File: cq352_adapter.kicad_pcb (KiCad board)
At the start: 2 copper layers, 2 parts, among them J1 FSI-150, X1 CQ352_SOCKET

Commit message: connector layout
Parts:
- added J2: FSI-150, spels:FSI-150-10-L-D-M-AD, F.Cu at (52.0, 135.0)
- added J3: FSI-150, spels:FSI-150-10-L-D-M-AD, F.Cu at (112.0, 205.0)
- added J4: FSI-150, spels:FSI-150-10-L-D-M-AD, F.Cu at (172.0, 135.0)
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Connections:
- J1 pad 1: Net-(J1-Pad1) -> (no net)
- J1 pad 10: Net-(J1-Pad10) -> (no net)
- J1 pad 100: Net-(J1-Pad100) -> (no net)
- J1 pad 11: Net-(J1-Pad11) -> (no net)
- J1 pad 12: Net-(J1-Pad12) -> (no net)
- J1 pad 13: Net-(J1-Pad13) -> (no net)
- J1 pad 14: Net-(J1-Pad14) -> (no net)
- J1 pad 15: Net-(J1-Pad15) -> (no net)
- J1 pad 16: Net-(J1-Pad16) -> (no net)
- J1 pad 17: Net-(J1-Pad17) -> (no net)
- J1 pad 18: Net-(J1-Pad18) -> (no net)
- J1 pad 19: Net-(J1-Pad19) -> (no net)
- J1 pad 2: Net-(J1-Pad2) -> (no net)
- J1 pad 20: Net-(J1-Pad20) -> (no net)
- J1 pad 21: Net-(J1-Pad21) -> (no net)
- J1 pad 22: Net-(J1-Pad22) -> (no net)
- J1 pad 23: Net-(J1-Pad23) -> (no net)
- J1 pad 24: Net-(J1-Pad24) -> (no net)
- J1 pad 25: Net-(J1-Pad25) -> (no net)
- J1 pad 26: Net-(J1-Pad26) -> (no net)
- J1 pad 27: Net-(J1-Pad27) -> (no net)
- J1 pad 28: Net-(J1-Pad28) -> (no net)
- J1 pad 29: Net-(J1-Pad29) -> (no net)
- J1 pad 3: Net-(J1-Pad3) -> (no net)
- J1 pad 30: Net-(J1-Pad30) -> (no net)
- J1 pad 31: Net-(J1-Pad31) -> (no net)
- J1 pad 32: Net-(J1-Pad32) -> (no net)
- J1 pad 33: Net-(J1-Pad33) -> (no net)
- J1 pad 34: Net-(J1-Pad34) -> (no net)
- J1 pad 35: Net-(J1-Pad35) -> (no net)
- J1 pad 36: Net-(J1-Pad36) -> (no net)
- J1 pad 37: Net-(J1-Pad37) -> (no net)
- J1 pad 38: Net-(J1-Pad38) -> (no net)
- J1 pad 39: Net-(J1-Pad39) -> (no net)
- J1 pad 4: Net-(J1-Pad4) -> (no net)
- J1 pad 40: Net-(J1-Pad40) -> (no net)
- J1 pad 41: Net-(J1-Pad41) -> (no net)
- J1 pad 42: Net-(J1-Pad42) -> (no net)
- J1 pad 43: Net-(J1-Pad43) -> (no net)
- J1 pad 44: Net-(J1-Pad44) -> (no net)
- J1 pad 45: Net-(J1-Pad45) -> (no net)
- J1 pad 46: Net-(J1-Pad46) -> (no net)
- J1 pad 47: Net-(J1-Pad47) -> (no net)
- J1 pad 48: Net-(J1-Pad48) -> (no net)
- J1 pad 49: Net-(J1-Pad49) -> (no net)
- J1 pad 5: Net-(J1-Pad5) -> (no net)
- J1 pad 50: Net-(J1-Pad50) -> (no net)
- J1 pad 51: Net-(J1-Pad51) -> (no net)
- J1 pad 52: Net-(J1-Pad52) -> (no net)
- J1 pad 53: Net-(J1-Pad53) -> (no net)
- J1 pad 54: Net-(J1-Pad54) -> (no net)
- J1 pad 55: Net-(J1-Pad55) -> (no net)
- J1 pad 56: Net-(J1-Pad56) -> (no net)
- J1 pad 57: Net-(J1-Pad57) -> (no net)
- J1 pad 58: Net-(J1-Pad58) -> (no net)
- J1 pad 59: Net-(J1-Pad59) -> (no net)
- J1 pad 6: Net-(J1-Pad6) -> (no net)
- J1 pad 60: Net-(J1-Pad60) -> (no net)
- J1 pad 61: Net-(J1-Pad61) -> (no net)
- J1 pad 62: Net-(J1-Pad62) -> (no net)
- J1 pad 63: Net-(J1-Pad63) -> (no net)
- J1 pad 64: Net-(J1-Pad64) -> (no net)
- J1 pad 65: Net-(J1-Pad65) -> (no net)
- J1 pad 66: Net-(J1-Pad66) -> (no net)
- J1 pad 67: Net-(J1-Pad67) -> (no net)
- J1 pad 68: Net-(J1-Pad68) -> (no net)
- J1 pad 69: Net-(J1-Pad69) -> (no net)
- J1 pad 7: Net-(J1-Pad7) -> (no net)
- J1 pad 70: Net-(J1-Pad70) -> (no net)
- J1 pad 71: Net-(J1-Pad71) -> (no net)
- J1 pad 72: Net-(J1-Pad72) -> (no net)
- J1 pad 73: Net-(J1-Pad73) -> (no net)
- J1 pad 74: Net-(J1-Pad74) -> (no net)
- J1 pad 75: Net-(J1-Pad75) -> (no net)
- J1 pad 76: Net-(J1-Pad76) -> (no net)
- J1 pad 77: Net-(J1-Pad77) -> (no net)
- J1 pad 78: Net-(J1-Pad78) -> (no net)
- J1 pad 79: Net-(J1-Pad79) -> (no net)
- J1 pad 8: Net-(J1-Pad8) -> (no net)
- J1 pad 80: Net-(J1-Pad80) -> (no net)
- J1 pad 81: Net-(J1-Pad81) -> (no net)
- J1 pad 82: Net-(J1-Pad82) -> (no net)
- J1 pad 83: Net-(J1-Pad83) -> (no net)
- J1 pad 84: Net-(J1-Pad84) -> (no net)
- J1 pad 85: Net-(J1-Pad85) -> (no net)
- J1 pad 86: Net-(J1-Pad86) -> (no net)
- J1 pad 87: Net-(J1-Pad87) -> (no net)
- J1 pad 88: Net-(J1-Pad88) -> (no net)
- J1 pad 89: Net-(J1-Pad89) -> (no net)
- J1 pad 9: Net-(J1-Pad9) -> (no net)
- J1 pad 90: Net-(J1-Pad90) -> (no net)
- J1 pad 91: Net-(J1-Pad91) -> (no net)
- J1 pad 92: Net-(J1-Pad92) -> (no net)
- J1 pad 93: Net-(J1-Pad93) -> (no net)
- J1 pad 94: Net-(J1-Pad94) -> (no net)
- J1 pad 95: Net-(J1-Pad95) -> (no net)
- J1 pad 96: Net-(J1-Pad96) -> (no net)
- J1 pad 97: Net-(J1-Pad97) -> (no net)
- J1 pad 98: Net-(J1-Pad98) -> (no net)
- J1 pad 99: Net-(J1-Pad99) -> (no net)
- J1 pad MH1: Net-(J1-PadMH1) -> (no net)
- J1 pad MH2: Net-(J1-PadMH2) -> (no net)
- J1 pad MH3: Net-(J1-PadMH3) -> (no net)
- X1 pad 1: Net-(X1-Pad1) -> (no net)
- X1 pad 10: Net-(X1-Pad10) -> (no net)
- X1 pad 100: Net-(X1-Pad100) -> (no net)
- X1 pad 101: Net-(X1-Pad101) -> (no net)
- X1 pad 102: Net-(X1-Pad102) -> (no net)
- X1 pad 103: Net-(X1-Pad103) -> (no net)
- X1 pad 104: Net-(X1-Pad104) -> (no net)
- X1 pad 105: Net-(X1-Pad105) -> (no net)
- X1 pad 106: Net-(X1-Pad106) -> (no net)
- X1 pad 107: Net-(X1-Pad107) -> (no net)
- X1 pad 108: Net-(X1-Pad108) -> (no net)
- X1 pad 109: Net-(X1-Pad109) -> (no net)
- X1 pad 11: Net-(X1-Pad11) -> (no net)
- X1 pad 110: Net-(X1-Pad110) -> (no net)
- X1 pad 111: Net-(X1-Pad111) -> (no net)
- X1 pad 112: Net-(X1-Pad112) -> (no net)
- X1 pad 113: Net-(X1-Pad113) -> (no net)
- X1 pad 114: Net-(X1-Pad114) -> (no net)
- X1 pad 115: Net-(X1-Pad115) -> (no net)
- X1 pad 116: Net-(X1-Pad116) -> (no net)
- X1 pad 117: Net-(X1-Pad117) -> (no net)
- X1 pad 118: Net-(X1-Pad118) -> (no net)
- X1 pad 119: Net-(X1-Pad119) -> (no net)
- X1 pad 12: Net-(X1-Pad12) -> (no net)
- X1 pad 120: Net-(X1-Pad120) -> (no net)
- X1 pad 121: Net-(X1-Pad121) -> (no net)
- X1 pad 122: Net-(X1-Pad122) -> (no net)
- X1 pad 123: Net-(X1-Pad123) -> (no net)
- X1 pad 124: Net-(X1-Pad124) -> (no net)
- X1 pad 125: Net-(X1-Pad125) -> (no net)
- X1 pad 126: Net-(X1-Pad126) -> (no net)
- X1 pad 127: Net-(X1-Pad127) -> (no net)
- X1 pad 128: Net-(X1-Pad128) -> (no net)
- X1 pad 129: Net-(X1-Pad129) -> (no net)
- X1 pad 13: Net-(X1-Pad13) -> (no net)
- X1 pad 130: Net-(X1-Pad130) -> (no net)
- X1 pad 131: Net-(X1-Pad131) -> (no net)
- X1 pad 132: Net-(X1-Pad132) -> (no net)
- X1 pad 133: Net-(X1-Pad133) -> (no net)
- X1 pad 134: Net-(X1-Pad134) -> (no net)
- X1 pad 135: Net-(X1-Pad135) -> (no net)
- X1 pad 136: Net-(X1-Pad136) -> (no net)
- X1 pad 137: Net-(X1-Pad137) -> (no net)
- X1 pad 138: Net-(X1-Pad138) -> (no net)
- X1 pad 139: Net-(X1-Pad139) -> (no net)
- X1 pad 14: Net-(X1-Pad14) -> (no net)
- X1 pad 140: Net-(X1-Pad140) -> (no net)
- X1 pad 141: Net-(X1-Pad141) -> (no net)
- X1 pad 142: Net-(X1-Pad142) -> (no net)
- X1 pad 143: Net-(X1-Pad143) -> (no net)
- X1 pad 144: Net-(X1-Pad144) -> (no net)
- X1 pad 145: Net-(X1-Pad145) -> (no net)
- X1 pad 146: Net-(X1-Pad146) -> (no net)
- X1 pad 147: Net-(X1-Pad147) -> (no net)
- X1 pad 148: Net-(X1-Pad148) -> (no net)
- X1 pad 149: Net-(X1-Pad149) -> (no net)
- X1 pad 15: Net-(X1-Pad15) -> (no net)
- X1 pad 150: Net-(X1-Pad150) -> (no net)
- X1 pad 151: Net-(X1-Pad151) -> (no net)
- X1 pad 152: Net-(X1-Pad152) -> (no net)
- X1 pad 153: Net-(X1-Pad153) -> (no net)
- X1 pad 154: Net-(X1-Pad154) -> (no net)
- X1 pad 155: Net-(X1-Pad155) -> (no net)
- X1 pad 156: Net-(X1-Pad156) -> (no net)
- X1 pad 157: Net-(X1-Pad157) -> (no net)
- X1 pad 158: Net-(X1-Pad158) -> (no net)
- X1 pad 159: Net-(X1-Pad159) -> (no net)
- X1 pad 16: Net-(X1-Pad16) -> (no net)
- X1 pad 160: Net-(X1-Pad160) -> (no net)
- X1 pad 161: Net-(X1-Pad161) -> (no net)
- X1 pad 162: Net-(X1-Pad162) -> (no net)
- X1 pad 163: Net-(X1-Pad163) -> (no net)
- X1 pad 164: Net-(X1-Pad164) -> (no net)
- X1 pad 165: Net-(X1-Pad165) -> (no net)
- X1 pad 166: Net-(X1-Pad166) -> (no net)
- X1 pad 167: Net-(X1-Pad167) -> (no net)
- X1 pad 168: Net-(X1-Pad168) -> (no net)
- X1 pad 169: Net-(X1-Pad169) -> (no net)
- X1 pad 17: Net-(X1-Pad17) -> (no net)
- X1 pad 170: Net-(X1-Pad170) -> (no net)
- X1 pad 171: Net-(X1-Pad171) -> (no net)
- X1 pad 172: Net-(X1-Pad172) -> (no net)
- X1 pad 173: Net-(X1-Pad173) -> (no net)
- X1 pad 174: Net-(X1-Pad174) -> (no net)
- X1 pad 175: Net-(X1-Pad175) -> (no net)
- X1 pad 176: Net-(X1-Pad176) -> (no net)
- X1 pad 177: Net-(X1-Pad177) -> (no net)
- X1 pad 178: Net-(X1-Pad178) -> (no net)
- X1 pad 179: Net-(X1-Pad179) -> (no net)
- X1 pad 18: Net-(X1-Pad18) -> (no net)
- X1 pad 180: Net-(X1-Pad180) -> (no net)
- X1 pad 181: Net-(X1-Pad181) -> (no net)
- X1 pad 182: Net-(X1-Pad182) -> (no net)
- X1 pad 183: Net-(X1-Pad183) -> (no net)
- X1 pad 184: Net-(X1-Pad184) -> (no net)
- X1 pad 185: Net-(X1-Pad185) -> (no net)
- X1 pad 186: Net-(X1-Pad186) -> (no net)
- X1 pad 187: Net-(X1-Pad187) -> (no net)
- X1 pad 188: Net-(X1-Pad188) -> (no net)
- X1 pad 189: Net-(X1-Pad189) -> (no net)
- X1 pad 19: Net-(X1-Pad19) -> (no net)
- X1 pad 190: Net-(X1-Pad190) -> (no net)
- X1 pad 191: Net-(X1-Pad191) -> (no net)
- X1 pad 192: Net-(X1-Pad192) -> (no net)
- X1 pad 193: Net-(X1-Pad193) -> (no net)
- X1 pad 194: Net-(X1-Pad194) -> (no net)
- X1 pad 195: Net-(X1-Pad195) -> (no net)
- X1 pad 196: Net-(X1-Pad196) -> (no net)
- X1 pad 197: Net-(X1-Pad197) -> (no net)
- X1 pad 198: Net-(X1-Pad198) -> (no net)
- X1 pad 199: Net-(X1-Pad199) -> (no net)
- X1 pad 2: Net-(X1-Pad2) -> (no net)
- X1 pad 20: Net-(X1-Pad20) -> (no net)
- X1 pad 200: Net-(X1-Pad200) -> (no net)
- X1 pad 201: Net-(X1-Pad201) -> (no net)
- X1 pad 202: Net-(X1-Pad202) -> (no net)
- X1 pad 203: Net-(X1-Pad203) -> (no net)
- X1 pad 204: Net-(X1-Pad204) -> (no net)
- X1 pad 205: Net-(X1-Pad205) -> (no net)
- X1 pad 206: Net-(X1-Pad206) -> (no net)
- X1 pad 207: Net-(X1-Pad207) -> (no net)
- X1 pad 208: Net-(X1-Pad208) -> (no net)
- X1 pad 209: Net-(X1-Pad209) -> (no net)
- X1 pad 21: Net-(X1-Pad21) -> (no net)
- X1 pad 210: Net-(X1-Pad210) -> (no net)
- X1 pad 211: Net-(X1-Pad211) -> (no net)
- X1 pad 212: Net-(X1-Pad212) -> (no net)
- X1 pad 213: Net-(X1-Pad213) -> (no net)
- X1 pad 214: Net-(X1-Pad214) -> (no net)
- X1 pad 215: Net-(X1-Pad215) -> (no net)
- X1 pad 216: Net-(X1-Pad216) -> (no net)
- X1 pad 217: Net-(X1-Pad217) -> (no net)
- X1 pad 218: Net-(X1-Pad218) -> (no net)
- X1 pad 219: Net-(X1-Pad219) -> (no net)
- X1 pad 22: Net-(X1-Pad22) -> (no net)
- X1 pad 220: Net-(X1-Pad220) -> (no net)
- X1 pad 221: Net-(X1-Pad221) -> (no net)
- X1 pad 222: Net-(X1-Pad222) -> (no net)
- X1 pad 223: Net-(X1-Pad223) -> (no net)
- X1 pad 224: Net-(X1-Pad224) -> (no net)
- X1 pad 225: Net-(X1-Pad225) -> (no net)
- X1 pad 226: Net-(X1-Pad226) -> (no net)
- X1 pad 227: Net-(X1-Pad227) -> (no net)
- X1 pad 228: Net-(X1-Pad228) -> (no net)
- X1 pad 229: Net-(X1-Pad229) -> (no net)
- X1 pad 23: Net-(X1-Pad23) -> (no net)
- X1 pad 230: Net-(X1-Pad230) -> (no net)
- X1 pad 231: Net-(X1-Pad231) -> (no net)
- X1 pad 232: Net-(X1-Pad232) -> (no net)
- X1 pad 233: Net-(X1-Pad233) -> (no net)
- X1 pad 234: Net-(X1-Pad234) -> (no net)
- X1 pad 235: Net-(X1-Pad235) -> (no net)
- X1 pad 236: Net-(X1-Pad236) -> (no net)
- X1 pad 237: Net-(X1-Pad237) -> (no net)
- X1 pad 238: Net-(X1-Pad238) -> (no net)
- X1 pad 239: Net-(X1-Pad239) -> (no net)
- X1 pad 24: Net-(X1-Pad24) -> (no net)
- X1 pad 240: Net-(X1-Pad240) -> (no net)
- X1 pad 241: Net-(X1-Pad241) -> (no net)
- X1 pad 242: Net-(X1-Pad242) -> (no net)
- X1 pad 243: Net-(X1-Pad243) -> (no net)
- X1 pad 244: Net-(X1-Pad244) -> (no net)
- X1 pad 245: Net-(X1-Pad245) -> (no net)
- X1 pad 246: Net-(X1-Pad246) -> (no net)
- X1 pad 247: Net-(X1-Pad247) -> (no net)
- X1 pad 248: Net-(X1-Pad248) -> (no net)
- X1 pad 249: Net-(X1-Pad249) -> (no net)
- X1 pad 25: Net-(X1-Pad25) -> (no net)
- X1 pad 250: Net-(X1-Pad250) -> (no net)
- X1 pad 251: Net-(X1-Pad251) -> (no net)
- X1 pad 252: Net-(X1-Pad252) -> (no net)
- X1 pad 253: Net-(X1-Pad253) -> (no net)
- X1 pad 254: Net-(X1-Pad254) -> (no net)
- X1 pad 255: Net-(X1-Pad255) -> (no net)
- X1 pad 256: Net-(X1-Pad256) -> (no net)
- X1 pad 257: Net-(X1-Pad257) -> (no net)
- X1 pad 258: Net-(X1-Pad258) -> (no net)
- X1 pad 259: Net-(X1-Pad259) -> (no net)
- X1 pad 26: Net-(X1-Pad26) -> (no net)
- X1 pad 260: Net-(X1-Pad260) -> (no net)
- X1 pad 261: Net-(X1-Pad261) -> (no net)
- X1 pad 262: Net-(X1-Pad262) -> (no net)
- X1 pad 263: Net-(X1-Pad263) -> (no net)
- X1 pad 264: Net-(X1-Pad264) -> (no net)
- X1 pad 265: Net-(X1-Pad265) -> (no net)
- X1 pad 266: Net-(X1-Pad266) -> (no net)
- X1 pad 267: Net-(X1-Pad267) -> (no net)
- X1 pad 268: Net-(X1-Pad268) -> (no net)
- X1 pad 269: Net-(X1-Pad269) -> (no net)
- X1 pad 27: Net-(X1-Pad27) -> (no net)
- X1 pad 270: Net-(X1-Pad270) -> (no net)
- X1 pad 271: Net-(X1-Pad271) -> (no net)
- X1 pad 272: Net-(X1-Pad272) -> (no net)
- X1 pad 273: Net-(X1-Pad273) -> (no net)
- X1 pad 274: Net-(X1-Pad274) -> (no net)
- X1 pad 275: Net-(X1-Pad275) -> (no net)
- X1 pad 276: Net-(X1-Pad276) -> (no net)
- X1 pad 277: Net-(X1-Pad277) -> (no net)
- X1 pad 278: Net-(X1-Pad278) -> (no net)
- X1 pad 279: Net-(X1-Pad279) -> (no net)
- X1 pad 28: Net-(X1-Pad28) -> (no net)
- X1 pad 280: Net-(X1-Pad280) -> (no net)
- X1 pad 281: Net-(X1-Pad281) -> (no net)
- X1 pad 282: Net-(X1-Pad282) -> (no net)
- X1 pad 283: Net-(X1-Pad283) -> (no net)
- X1 pad 284: Net-(X1-Pad284) -> (no net)
- X1 pad 285: Net-(X1-Pad285) -> (no net)
- X1 pad 286: Net-(X1-Pad286) -> (no net)
- X1 pad 287: Net-(X1-Pad287) -> (no net)
- X1 pad 288: Net-(X1-Pad288) -> (no net)
- X1 pad 289: Net-(X1-Pad289) -> (no net)
- X1 pad 29: Net-(X1-Pad29) -> (no net)
- X1 pad 290: Net-(X1-Pad290) -> (no net)
- X1 pad 291: Net-(X1-Pad291) -> (no net)
- X1 pad 292: Net-(X1-Pad292) -> (no net)
- X1 pad 293: Net-(X1-Pad293) -> (no net)
- X1 pad 294: Net-(X1-Pad294) -> (no net)
- X1 pad 295: Net-(X1-Pad295) -> (no net)
- X1 pad 296: Net-(X1-Pad296) -> (no net)
- X1 pad 297: Net-(X1-Pad297) -> (no net)
- X1 pad 298: Net-(X1-Pad298) -> (no net)
- X1 pad 299: Net-(X1-Pad299) -> (no net)
- X1 pad 3: Net-(X1-Pad3) -> (no net)
- X1 pad 30: Net-(X1-Pad30) -> (no net)
- X1 pad 300: Net-(X1-Pad300) -> (no net)
- X1 pad 301: Net-(X1-Pad301) -> (no net)
- X1 pad 302: Net-(X1-Pad302) -> (no net)
- X1 pad 303: Net-(X1-Pad303) -> (no net)
- X1 pad 304: Net-(X1-Pad304) -> (no net)
- X1 pad 305: Net-(X1-Pad305) -> (no net)
- X1 pad 306: Net-(X1-Pad306) -> (no net)
- X1 pad 307: Net-(X1-Pad307) -> (no net)
- X1 pad 308: Net-(X1-Pad308) -> (no net)
- X1 pad 309: Net-(X1-Pad309) -> (no net)
- X1 pad 31: Net-(X1-Pad31) -> (no net)
- X1 pad 310: Net-(X1-Pad310) -> (no net)
- X1 pad 311: Net-(X1-Pad311) -> (no net)
- X1 pad 312: Net-(X1-Pad312) -> (no net)
- X1 pad 313: Net-(X1-Pad313) -> (no net)
- X1 pad 314: Net-(X1-Pad314) -> (no net)
- X1 pad 315: Net-(X1-Pad315) -> (no net)
- X1 pad 316: Net-(X1-Pad316) -> (no net)
- X1 pad 317: Net-(X1-Pad317) -> (no net)
- X1 pad 318: Net-(X1-Pad318) -> (no net)
- X1 pad 319: Net-(X1-Pad319) -> (no net)
- X1 pad 32: Net-(X1-Pad32) -> (no net)
- X1 pad 320: Net-(X1-Pad320) -> (no net)
- X1 pad 321: Net-(X1-Pad321) -> (no net)
- X1 pad 322: Net-(X1-Pad322) -> (no net)
- X1 pad 323: Net-(X1-Pad323) -> (no net)
- X1 pad 324: Net-(X1-Pad324) -> (no net)
- X1 pad 325: Net-(X1-Pad325) -> (no net)
- X1 pad 326: Net-(X1-Pad326) -> (no net)
- X1 pad 327: Net-(X1-Pad327) -> (no net)
- X1 pad 328: Net-(X1-Pad328) -> (no net)
- X1 pad 329: Net-(X1-Pad329) -> (no net)
- X1 pad 33: Net-(X1-Pad33) -> (no net)
- X1 pad 330: Net-(X1-Pad330) -> (no net)
- X1 pad 331: Net-(X1-Pad331) -> (no net)
- X1 pad 332: Net-(X1-Pad332) -> (no net)
- X1 pad 333: Net-(X1-Pad333) -> (no net)
- X1 pad 334: Net-(X1-Pad334) -> (no net)
- X1 pad 335: Net-(X1-Pad335) -> (no net)
- X1 pad 336: Net-(X1-Pad336) -> (no net)
- X1 pad 337: Net-(X1-Pad337) -> (no net)
- X1 pad 338: Net-(X1-Pad338) -> (no net)
- X1 pad 339: Net-(X1-Pad339) -> (no net)
- X1 pad 34: Net-(X1-Pad34) -> (no net)
- X1 pad 340: Net-(X1-Pad340) -> (no net)
- X1 pad 341: Net-(X1-Pad341) -> (no net)
- X1 pad 342: Net-(X1-Pad342) -> (no net)
- X1 pad 343: Net-(X1-Pad343) -> (no net)
- X1 pad 344: Net-(X1-Pad344) -> (no net)
- X1 pad 345: Net-(X1-Pad345) -> (no net)
- X1 pad 346: Net-(X1-Pad346) -> (no net)
- X1 pad 347: Net-(X1-Pad347) -> (no net)
- X1 pad 348: Net-(X1-Pad348) -> (no net)
- X1 pad 349: Net-(X1-Pad349) -> (no net)
- X1 pad 35: Net-(X1-Pad35) -> (no net)
- X1 pad 350: Net-(X1-Pad350) -> (no net)
- X1 pad 351: Net-(X1-Pad351) -> (no net)
- X1 pad 352: Net-(X1-Pad352) -> (no net)
- X1 pad 36: Net-(X1-Pad36) -> (no net)
- X1 pad 37: Net-(X1-Pad37) -> (no net)
- X1 pad 38: Net-(X1-Pad38) -> (no net)
- X1 pad 39: Net-(X1-Pad39) -> (no net)
- X1 pad 4: Net-(X1-Pad4) -> (no net)
- X1 pad 40: Net-(X1-Pad40) -> (no net)
- X1 pad 41: Net-(X1-Pad41) -> (no net)
- X1 pad 42: Net-(X1-Pad42) -> (no net)
- X1 pad 43: Net-(X1-Pad43) -> (no net)
- X1 pad 44: Net-(X1-Pad44) -> (no net)
- X1 pad 45: Net-(X1-Pad45) -> (no net)
- X1 pad 46: Net-(X1-Pad46) -> (no net)
- X1 pad 47: Net-(X1-Pad47) -> (no net)
- X1 pad 48: Net-(X1-Pad48) -> (no net)
- X1 pad 49: Net-(X1-Pad49) -> (no net)
- X1 pad 5: Net-(X1-Pad5) -> (no net)
- X1 pad 50: Net-(X1-Pad50) -> (no net)
- X1 pad 51: Net-(X1-Pad51) -> (no net)
- X1 pad 52: Net-(X1-Pad52) -> (no net)
- X1 pad 53: Net-(X1-Pad53) -> (no net)
- X1 pad 54: Net-(X1-Pad54) -> (no net)
- X1 pad 55: Net-(X1-Pad55) -> (no net)
- X1 pad 56: Net-(X1-Pad56) -> (no net)
- X1 pad 57: Net-(X1-Pad57) -> (no net)
- X1 pad 58: Net-(X1-Pad58) -> (no net)
- X1 pad 59: Net-(X1-Pad59) -> (no net)
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
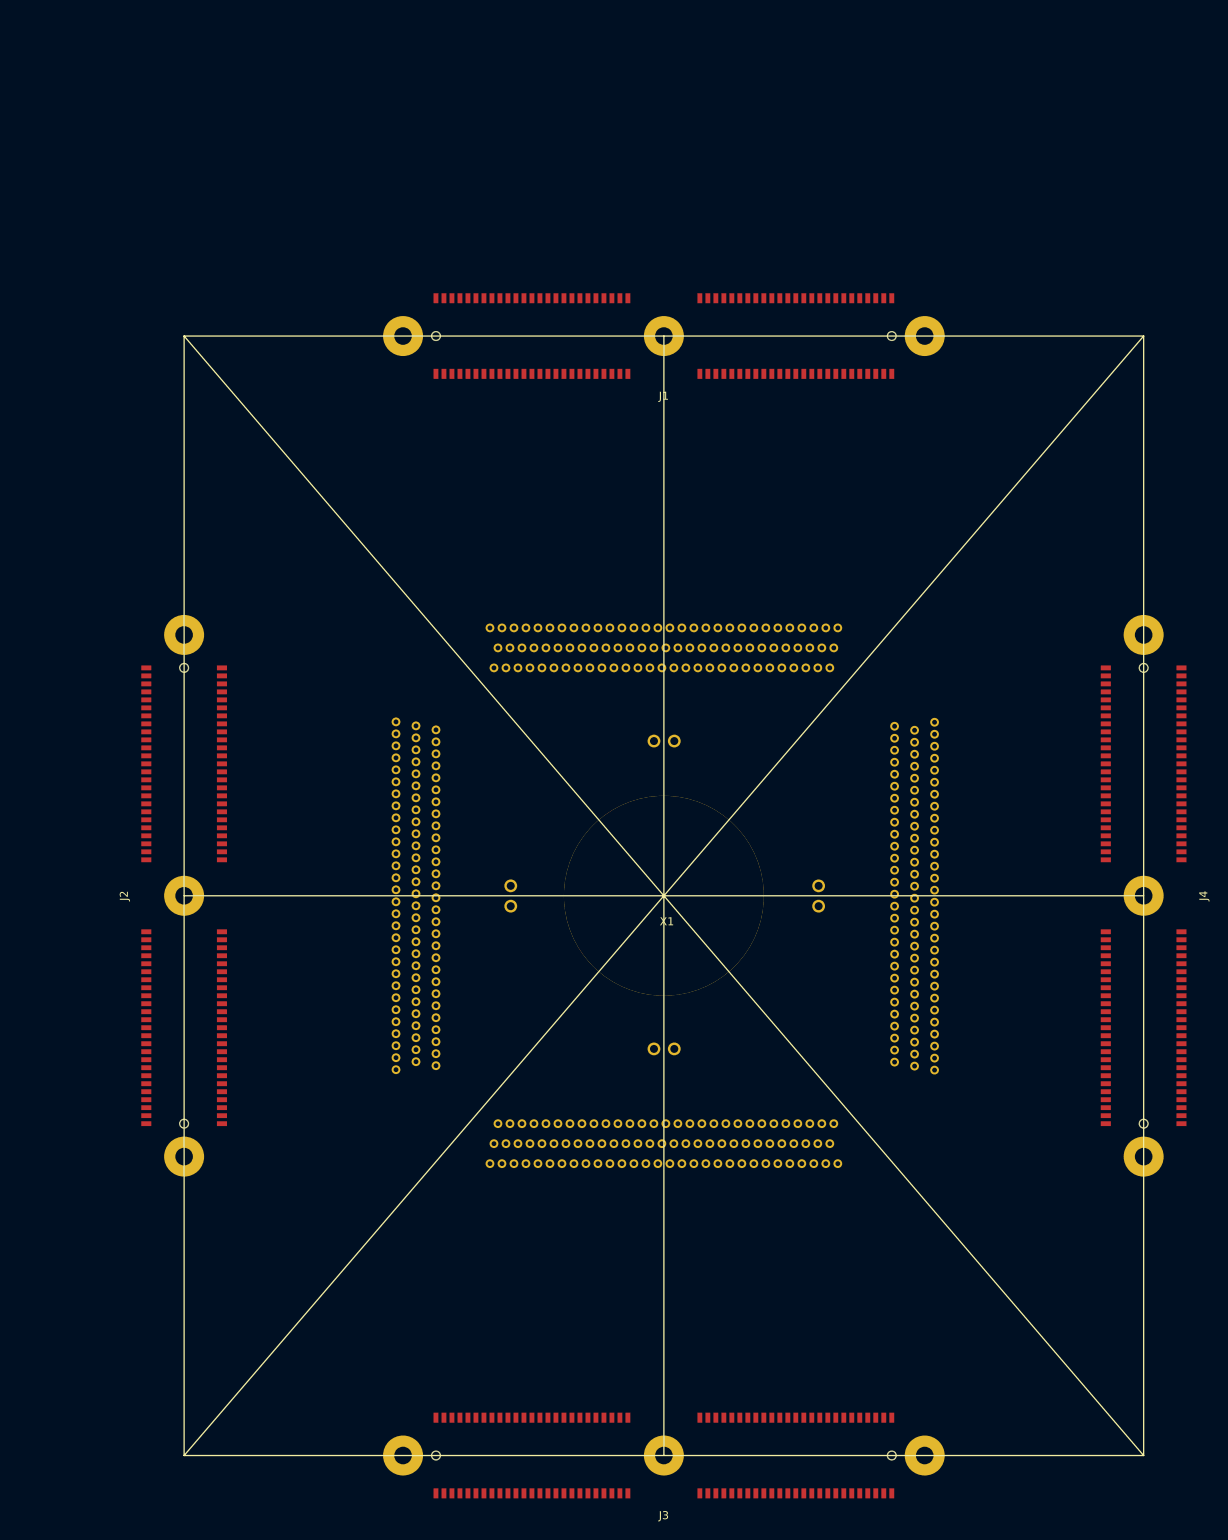
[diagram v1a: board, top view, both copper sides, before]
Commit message: routing signals
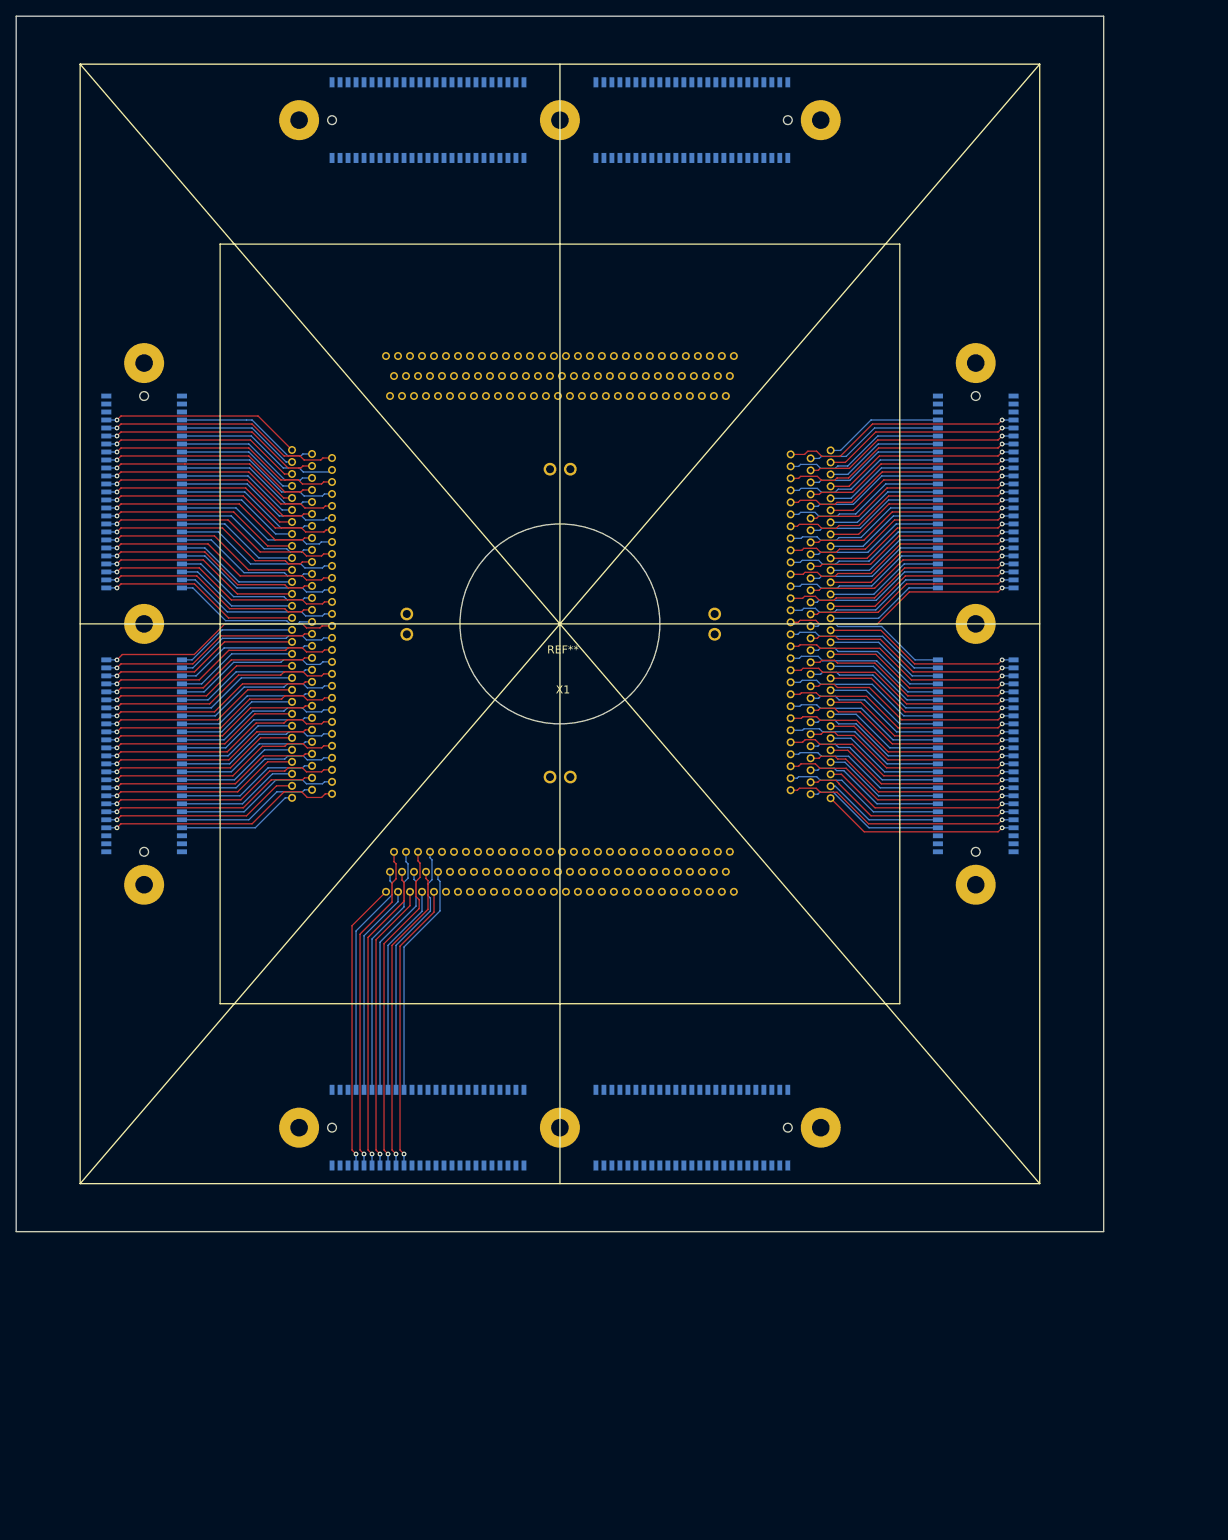
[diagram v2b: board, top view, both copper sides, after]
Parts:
- J1, J2, J3, J4: moved to B.Cu
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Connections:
- J1 pad 1: (no net) -> Net-(J1-Pad1)
- J1 pad 10: (no net) -> /4
- J1 pad 100: (no net) -> Net-(J1-Pad100)
- J1 pad 11: (no net) -> /5
- J1 pad 12: (no net) -> /6
- J1 pad 13: (no net) -> /7
- J1 pad 14: (no net) -> /8
- J1 pad 15: (no net) -> /9
- J1 pad 16: (no net) -> /10
- J1 pad 17: (no net) -> /11
- J1 pad 18: (no net) -> /12
- J1 pad 19: (no net) -> /13
- J1 pad 2: (no net) -> Net-(J1-Pad2)
- J1 pad 20: (no net) -> /14
- J1 pad 21: (no net) -> /15
- J1 pad 22: (no net) -> /16
- J1 pad 23: (no net) -> /17
- J1 pad 24: (no net) -> /18
- J1 pad 25: (no net) -> /19
- J1 pad 26: (no net) -> /20
- J1 pad 27: (no net) -> /21
- J1 pad 28: (no net) -> /22
- J1 pad 29: (no net) -> /23
- J1 pad 3: (no net) -> Net-(J1-Pad3)
- J1 pad 30: (no net) -> /24
- J1 pad 31: (no net) -> /25
- J1 pad 32: (no net) -> /26
- J1 pad 33: (no net) -> /27
- J1 pad 34: (no net) -> /28
- J1 pad 35: (no net) -> /29
- J1 pad 36: (no net) -> /30
- J1 pad 37: (no net) -> /31
- J1 pad 38: (no net) -> /32
- J1 pad 39: (no net) -> /33
- J1 pad 4: (no net) -> Net-(J1-Pad4)
- J1 pad 40: (no net) -> /34
- J1 pad 41: (no net) -> /35
- J1 pad 42: (no net) -> /36
- J1 pad 43: (no net) -> /37
- J1 pad 44: (no net) -> /38
- J1 pad 45: (no net) -> /39
- J1 pad 46: (no net) -> /40
- J1 pad 47: (no net) -> /41
- J1 pad 48: (no net) -> /42
- J1 pad 49: (no net) -> /43
- J1 pad 5: (no net) -> Net-(J1-Pad5)
- J1 pad 50: (no net) -> /44
- J1 pad 51: (no net) -> /45
- J1 pad 52: (no net) -> /46
- J1 pad 53: (no net) -> /47
- J1 pad 54: (no net) -> /48
- J1 pad 55: (no net) -> /49
- J1 pad 56: (no net) -> /50
- J1 pad 57: (no net) -> /51
- J1 pad 58: (no net) -> /52
- J1 pad 59: (no net) -> /53
- J1 pad 6: (no net) -> Net-(J1-Pad6)
- J1 pad 60: (no net) -> /54
- J1 pad 61: (no net) -> /55
- J1 pad 62: (no net) -> /56
- J1 pad 63: (no net) -> /57
- J1 pad 64: (no net) -> /58
- J1 pad 65: (no net) -> /59
- J1 pad 66: (no net) -> /60
- J1 pad 67: (no net) -> /61
- J1 pad 68: (no net) -> /62
- J1 pad 69: (no net) -> /63
- J1 pad 7: (no net) -> /1
- J1 pad 70: (no net) -> /64
- J1 pad 71: (no net) -> /65
- J1 pad 72: (no net) -> /66
- J1 pad 73: (no net) -> /67
- J1 pad 74: (no net) -> /68
- J1 pad 75: (no net) -> /69
- J1 pad 76: (no net) -> /70
- J1 pad 77: (no net) -> /71
- J1 pad 78: (no net) -> /72
- J1 pad 79: (no net) -> /73
- J1 pad 8: (no net) -> /2
- J1 pad 80: (no net) -> /74
- J1 pad 81: (no net) -> /75
- J1 pad 82: (no net) -> /76
- J1 pad 83: (no net) -> /77
- J1 pad 84: (no net) -> /78
- J1 pad 85: (no net) -> /79
- J1 pad 86: (no net) -> /80
- J1 pad 87: (no net) -> /81
- J1 pad 88: (no net) -> /82
- J1 pad 89: (no net) -> /83
- J1 pad 9: (no net) -> /3
- J1 pad 90: (no net) -> /84
- J1 pad 91: (no net) -> /85
- J1 pad 92: (no net) -> /86
- J1 pad 93: (no net) -> /87
- J1 pad 94: (no net) -> /88
- J1 pad 95: (no net) -> Net-(J1-Pad95)
- J1 pad 96: (no net) -> Net-(J1-Pad96)
- J1 pad 97: (no net) -> Net-(J1-Pad97)
- J1 pad 98: (no net) -> Net-(J1-Pad98)
- J1 pad 99: (no net) -> Net-(J1-Pad99)
- J1 pad MH1: (no net) -> Net-(J1-PadMH1)
- J1 pad MH2: (no net) -> Net-(J1-PadMH2)
- J1 pad MH3: (no net) -> Net-(J1-PadMH3)
- J2 pad 1: (no net) -> Net-(J2-Pad1)
- J2 pad 10: (no net) -> /92
- J2 pad 100: (no net) -> Net-(J2-Pad100)
- J2 pad 11: (no net) -> /93
- J2 pad 12: (no net) -> /94
- J2 pad 13: (no net) -> /95
- J2 pad 14: (no net) -> /96
- J2 pad 15: (no net) -> /97
- J2 pad 16: (no net) -> /98
- J2 pad 17: (no net) -> /99
- J2 pad 18: (no net) -> /100
- J2 pad 19: (no net) -> /101
- J2 pad 2: (no net) -> Net-(J2-Pad2)
- J2 pad 20: (no net) -> /102
- J2 pad 21: (no net) -> /103
- J2 pad 22: (no net) -> /104
- J2 pad 23: (no net) -> /105
- J2 pad 24: (no net) -> /106
- J2 pad 25: (no net) -> /107
- J2 pad 26: (no net) -> /108
- J2 pad 27: (no net) -> /109
- J2 pad 28: (no net) -> /110
- J2 pad 29: (no net) -> /111
- J2 pad 3: (no net) -> Net-(J2-Pad3)
- J2 pad 30: (no net) -> /112
- J2 pad 31: (no net) -> /113
- J2 pad 32: (no net) -> /114
- J2 pad 33: (no net) -> /115
- J2 pad 34: (no net) -> /116
- J2 pad 35: (no net) -> /117
- J2 pad 36: (no net) -> /118
- J2 pad 37: (no net) -> /119
- J2 pad 38: (no net) -> /120
- J2 pad 39: (no net) -> /121
- J2 pad 4: (no net) -> Net-(J2-Pad4)
- J2 pad 40: (no net) -> /122
- J2 pad 41: (no net) -> /123
- J2 pad 42: (no net) -> /124
- J2 pad 43: (no net) -> /125
- J2 pad 44: (no net) -> /126
- J2 pad 45: (no net) -> /127
- J2 pad 46: (no net) -> /128
- J2 pad 47: (no net) -> /129
- J2 pad 48: (no net) -> /130
- J2 pad 49: (no net) -> /131
- J2 pad 5: (no net) -> Net-(J2-Pad5)
- J2 pad 50: (no net) -> /132
- J2 pad 51: (no net) -> /133
- J2 pad 52: (no net) -> /134
- J2 pad 53: (no net) -> /135
- J2 pad 54: (no net) -> /136
- J2 pad 55: (no net) -> /137
- J2 pad 56: (no net) -> /138
- J2 pad 57: (no net) -> /139
- J2 pad 58: (no net) -> /140
- J2 pad 59: (no net) -> /141
- J2 pad 6: (no net) -> Net-(J2-Pad6)
- J2 pad 60: (no net) -> /142
- J2 pad 61: (no net) -> /143
- J2 pad 62: (no net) -> /144
- J2 pad 63: (no net) -> /145
- J2 pad 64: (no net) -> /146
- J2 pad 65: (no net) -> /147
- J2 pad 66: (no net) -> /148
- J2 pad 67: (no net) -> /149
- J2 pad 68: (no net) -> /150
- J2 pad 69: (no net) -> /151
- J2 pad 7: (no net) -> /89
- J2 pad 70: (no net) -> /152
- J2 pad 71: (no net) -> /153
- J2 pad 72: (no net) -> /154
- J2 pad 73: (no net) -> /155
- J2 pad 74: (no net) -> /156
- J2 pad 75: (no net) -> /157
- J2 pad 76: (no net) -> /158
- J2 pad 77: (no net) -> /159
- J2 pad 78: (no net) -> /160
- J2 pad 79: (no net) -> /161
- J2 pad 8: (no net) -> /90
- J2 pad 80: (no net) -> /162
- J2 pad 81: (no net) -> /163
- J2 pad 82: (no net) -> /164
- J2 pad 83: (no net) -> /165
- J2 pad 84: (no net) -> /166
- J2 pad 85: (no net) -> /167
- J2 pad 86: (no net) -> /168
- J2 pad 87: (no net) -> /169
- J2 pad 88: (no net) -> /170
- J2 pad 89: (no net) -> /171
- J2 pad 9: (no net) -> /91
- J2 pad 90: (no net) -> /172
- J2 pad 91: (no net) -> /173
- J2 pad 92: (no net) -> /174
- J2 pad 93: (no net) -> /175
- J2 pad 94: (no net) -> /176
- J2 pad 95: (no net) -> Net-(J2-Pad95)
- J2 pad 96: (no net) -> Net-(J2-Pad96)
- J2 pad 97: (no net) -> Net-(J2-Pad97)
- J2 pad 98: (no net) -> Net-(J2-Pad98)
- J2 pad 99: (no net) -> Net-(J2-Pad99)
- J2 pad MH1: (no net) -> Net-(J2-PadMH1)
- J2 pad MH2: (no net) -> Net-(J2-PadMH2)
- J2 pad MH3: (no net) -> Net-(J2-PadMH3)
- J3 pad 1: (no net) -> Net-(J3-Pad1)
- J3 pad 10: (no net) -> /180
- J3 pad 100: (no net) -> Net-(J3-Pad100)
- J3 pad 11: (no net) -> /181
- J3 pad 12: (no net) -> /182
- J3 pad 13: (no net) -> /183
- J3 pad 14: (no net) -> /184
- J3 pad 15: (no net) -> /185
- J3 pad 16: (no net) -> /186
- J3 pad 17: (no net) -> /187
- J3 pad 18: (no net) -> /188
- J3 pad 19: (no net) -> /189
- J3 pad 2: (no net) -> Net-(J3-Pad2)
- J3 pad 20: (no net) -> /190
- J3 pad 21: (no net) -> /191
- J3 pad 22: (no net) -> /192
- J3 pad 23: (no net) -> /193
- J3 pad 24: (no net) -> /194
- J3 pad 25: (no net) -> /195
- J3 pad 26: (no net) -> /196
- J3 pad 27: (no net) -> /197
- J3 pad 28: (no net) -> /198
- J3 pad 29: (no net) -> /199
- J3 pad 3: (no net) -> Net-(J3-Pad3)
- J3 pad 30: (no net) -> /200
- J3 pad 31: (no net) -> /201
- J3 pad 32: (no net) -> /202
- J3 pad 33: (no net) -> /203
- J3 pad 34: (no net) -> /204
- J3 pad 35: (no net) -> /205
- J3 pad 36: (no net) -> /206
- J3 pad 37: (no net) -> /207
- J3 pad 38: (no net) -> /208
- J3 pad 39: (no net) -> /209
- J3 pad 4: (no net) -> Net-(J3-Pad4)
- J3 pad 40: (no net) -> /210
- J3 pad 41: (no net) -> /211
- J3 pad 42: (no net) -> /212
- J3 pad 43: (no net) -> /213
- J3 pad 44: (no net) -> /214
- J3 pad 45: (no net) -> /215
- J3 pad 46: (no net) -> /216
- J3 pad 47: (no net) -> /217
- J3 pad 48: (no net) -> /218
- J3 pad 49: (no net) -> /219
- J3 pad 5: (no net) -> Net-(J3-Pad5)
- J3 pad 50: (no net) -> /220
- J3 pad 51: (no net) -> /221
- J3 pad 52: (no net) -> /222
- J3 pad 53: (no net) -> /223
- J3 pad 54: (no net) -> /224
- J3 pad 55: (no net) -> /225
- J3 pad 56: (no net) -> /226
- J3 pad 57: (no net) -> /227
- J3 pad 58: (no net) -> /228
- J3 pad 59: (no net) -> /229
- J3 pad 6: (no net) -> Net-(J3-Pad6)
- J3 pad 60: (no net) -> /230
- J3 pad 61: (no net) -> /231
- J3 pad 62: (no net) -> /232
- J3 pad 63: (no net) -> /233
- J3 pad 64: (no net) -> /234
- J3 pad 65: (no net) -> /235
- J3 pad 66: (no net) -> /236
- J3 pad 67: (no net) -> /237
- J3 pad 68: (no net) -> /238
- J3 pad 69: (no net) -> /239
- J3 pad 7: (no net) -> /177
- J3 pad 70: (no net) -> /240
- J3 pad 71: (no net) -> /241
- J3 pad 72: (no net) -> /242
- J3 pad 73: (no net) -> /243
- J3 pad 74: (no net) -> /244
- J3 pad 75: (no net) -> /245
- J3 pad 76: (no net) -> /246
- J3 pad 77: (no net) -> /247
- J3 pad 78: (no net) -> /248
- J3 pad 79: (no net) -> /249
- J3 pad 8: (no net) -> /178
- J3 pad 80: (no net) -> /250
- J3 pad 81: (no net) -> /251
- J3 pad 82: (no net) -> /252
- J3 pad 83: (no net) -> /253
- J3 pad 84: (no net) -> /254
- J3 pad 85: (no net) -> /255
- J3 pad 86: (no net) -> /256
- J3 pad 87: (no net) -> /257
- J3 pad 88: (no net) -> /258
- J3 pad 89: (no net) -> /259
- J3 pad 9: (no net) -> /179
- J3 pad 90: (no net) -> /260
- J3 pad 91: (no net) -> /261
- J3 pad 92: (no net) -> /262
- J3 pad 93: (no net) -> /263
- J3 pad 94: (no net) -> /264
- J3 pad 95: (no net) -> Net-(J3-Pad95)
- J3 pad 96: (no net) -> Net-(J3-Pad96)
- J3 pad 97: (no net) -> Net-(J3-Pad97)
- J3 pad 98: (no net) -> Net-(J3-Pad98)
- J3 pad 99: (no net) -> Net-(J3-Pad99)
- J3 pad MH1: (no net) -> Net-(J3-PadMH1)
- J3 pad MH2: (no net) -> Net-(J3-PadMH2)
- J3 pad MH3: (no net) -> Net-(J3-PadMH3)
- J4 pad 1: (no net) -> Net-(J4-Pad1)
- J4 pad 10: (no net) -> /268
- J4 pad 100: (no net) -> Net-(J4-Pad100)
- J4 pad 11: (no net) -> /269
- J4 pad 12: (no net) -> /270
- J4 pad 13: (no net) -> /271
- J4 pad 14: (no net) -> /272
- J4 pad 15: (no net) -> /273
- J4 pad 16: (no net) -> /274
- J4 pad 17: (no net) -> /275
- J4 pad 18: (no net) -> /276
- J4 pad 19: (no net) -> /277
- J4 pad 2: (no net) -> Net-(J4-Pad2)
- J4 pad 20: (no net) -> /278
- J4 pad 21: (no net) -> /279
- J4 pad 22: (no net) -> /280
- J4 pad 23: (no net) -> /281
- J4 pad 24: (no net) -> /282
- J4 pad 25: (no net) -> /283
- J4 pad 26: (no net) -> /284
- J4 pad 27: (no net) -> /285
- J4 pad 28: (no net) -> /286
- J4 pad 29: (no net) -> /287
- J4 pad 3: (no net) -> Net-(J4-Pad3)
- J4 pad 30: (no net) -> /288
- J4 pad 31: (no net) -> /289
- J4 pad 32: (no net) -> /290
- J4 pad 33: (no net) -> /291
- J4 pad 34: (no net) -> /292
- J4 pad 35: (no net) -> /293
- J4 pad 36: (no net) -> /294
- J4 pad 37: (no net) -> /295
- J4 pad 38: (no net) -> /296
- J4 pad 39: (no net) -> /297
- J4 pad 4: (no net) -> Net-(J4-Pad4)
- J4 pad 40: (no net) -> /298
- J4 pad 41: (no net) -> /299
- J4 pad 42: (no net) -> /300
- J4 pad 43: (no net) -> /301
- J4 pad 44: (no net) -> /302
- J4 pad 45: (no net) -> /303
- J4 pad 46: (no net) -> /304
- J4 pad 47: (no net) -> /305
- J4 pad 48: (no net) -> /306
- J4 pad 49: (no net) -> /307
- J4 pad 5: (no net) -> Net-(J4-Pad5)
- J4 pad 50: (no net) -> /308
- J4 pad 51: (no net) -> /309
- J4 pad 52: (no net) -> /310
- J4 pad 53: (no net) -> /311
- J4 pad 54: (no net) -> /312
- J4 pad 55: (no net) -> /313
- J4 pad 56: (no net) -> /314
- J4 pad 57: (no net) -> /315
- J4 pad 58: (no net) -> /316
- J4 pad 59: (no net) -> /317
- J4 pad 6: (no net) -> Net-(J4-Pad6)
- J4 pad 60: (no net) -> /318
- J4 pad 61: (no net) -> /319
- J4 pad 62: (no net) -> /320
- J4 pad 63: (no net) -> /321
- J4 pad 64: (no net) -> /322
- J4 pad 65: (no net) -> /323
- J4 pad 66: (no net) -> /324
- J4 pad 67: (no net) -> /325
- J4 pad 68: (no net) -> /326
- J4 pad 69: (no net) -> /327
- J4 pad 7: (no net) -> /265
- J4 pad 70: (no net) -> /328
- J4 pad 71: (no net) -> /329
- J4 pad 72: (no net) -> /330
- J4 pad 73: (no net) -> /331
- J4 pad 74: (no net) -> /332
- J4 pad 75: (no net) -> /333
- J4 pad 76: (no net) -> /334
- J4 pad 77: (no net) -> /335
- J4 pad 78: (no net) -> /336
- J4 pad 79: (no net) -> /337
- J4 pad 8: (no net) -> /266
- J4 pad 80: (no net) -> /338
- J4 pad 81: (no net) -> /339
- J4 pad 82: (no net) -> /340
- J4 pad 83: (no net) -> /341
- J4 pad 84: (no net) -> /342
- J4 pad 85: (no net) -> /343
- J4 pad 86: (no net) -> /344
- J4 pad 87: (no net) -> /345
- J4 pad 88: (no net) -> /346
- J4 pad 89: (no net) -> /347
- J4 pad 9: (no net) -> /267
- J4 pad 90: (no net) -> /348
- J4 pad 91: (no net) -> /349
- J4 pad 92: (no net) -> /350
- J4 pad 93: (no net) -> /351
- J4 pad 94: (no net) -> /352
- J4 pad 95: (no net) -> Net-(J4-Pad95)
- J4 pad 96: (no net) -> Net-(J4-Pad96)
- J4 pad 97: (no net) -> Net-(J4-Pad97)
- J4 pad 98: (no net) -> Net-(J4-Pad98)
- J4 pad 99: (no net) -> Net-(J4-Pad99)
- J4 pad MH1: (no net) -> Net-(J4-PadMH1)
- J4 pad MH2: (no net) -> Net-(J4-PadMH2)
- J4 pad MH3: (no net) -> Net-(J4-PadMH3)
- X1 pad 1: (no net) -> /1
- X1 pad 10: (no net) -> /10
- X1 pad 100: (no net) -> /100
- X1 pad 101: (no net) -> /101
- X1 pad 102: (no net) -> /102
- X1 pad 103: (no net) -> /103
- X1 pad 104: (no net) -> /104
- X1 pad 105: (no net) -> /105
- X1 pad 106: (no net) -> /106
- X1 pad 107: (no net) -> /107
- X1 pad 108: (no net) -> /108
- X1 pad 109: (no net) -> /109
- X1 pad 11: (no net) -> /11
- X1 pad 110: (no net) -> /110
- X1 pad 111: (no net) -> /111
- X1 pad 112: (no net) -> /112
- X1 pad 113: (no net) -> /113
- X1 pad 114: (no net) -> /114
- X1 pad 115: (no net) -> /115
- X1 pad 116: (no net) -> /116
- X1 pad 117: (no net) -> /117
- X1 pad 118: (no net) -> /118
- X1 pad 119: (no net) -> /119
- X1 pad 12: (no net) -> /12
- X1 pad 120: (no net) -> /120
- X1 pad 121: (no net) -> /121
- X1 pad 122: (no net) -> /122
- X1 pad 123: (no net) -> /123
- X1 pad 124: (no net) -> /124
- X1 pad 125: (no net) -> /125
- X1 pad 126: (no net) -> /126
- X1 pad 127: (no net) -> /127
- X1 pad 128: (no net) -> /128
- X1 pad 129: (no net) -> /129
- X1 pad 13: (no net) -> /13
- X1 pad 130: (no net) -> /130
- X1 pad 131: (no net) -> /131
- X1 pad 132: (no net) -> /132
- X1 pad 133: (no net) -> /133
- X1 pad 134: (no net) -> /134
- X1 pad 135: (no net) -> /135
- X1 pad 136: (no net) -> /136
- X1 pad 137: (no net) -> /137
- X1 pad 138: (no net) -> /138
- X1 pad 139: (no net) -> /139
- X1 pad 14: (no net) -> /14
- X1 pad 140: (no net) -> /140
- X1 pad 141: (no net) -> /141
- X1 pad 142: (no net) -> /142
- X1 pad 143: (no net) -> /143
- X1 pad 144: (no net) -> /144
- X1 pad 145: (no net) -> /145
- X1 pad 146: (no net) -> /146
- X1 pad 147: (no net) -> /147
- X1 pad 148: (no net) -> /148
- X1 pad 149: (no net) -> /149
- X1 pad 15: (no net) -> /15
- X1 pad 150: (no net) -> /150
- X1 pad 151: (no net) -> /151
- X1 pad 152: (no net) -> /152
- X1 pad 153: (no net) -> /153
- X1 pad 154: (no net) -> /154
- X1 pad 155: (no net) -> /155
- X1 pad 156: (no net) -> /156
- X1 pad 157: (no net) -> /157
- X1 pad 158: (no net) -> /158
- X1 pad 159: (no net) -> /159
- X1 pad 16: (no net) -> /16
- X1 pad 160: (no net) -> /160
- X1 pad 161: (no net) -> /161
- X1 pad 162: (no net) -> /162
- X1 pad 163: (no net) -> /163
- X1 pad 164: (no net) -> /164
- X1 pad 165: (no net) -> /165
- X1 pad 166: (no net) -> /166
- X1 pad 167: (no net) -> /167
- X1 pad 168: (no net) -> /168
- X1 pad 169: (no net) -> /169
- X1 pad 17: (no net) -> /17
- X1 pad 170: (no net) -> /170
- X1 pad 171: (no net) -> /171
- X1 pad 172: (no net) -> /172
- X1 pad 173: (no net) -> /173
- X1 pad 174: (no net) -> /174
- X1 pad 175: (no net) -> /175
- X1 pad 176: (no net) -> /176
- X1 pad 177: (no net) -> /177
- X1 pad 178: (no net) -> /178
- X1 pad 179: (no net) -> /179
- X1 pad 18: (no net) -> /18
- X1 pad 180: (no net) -> /180
- X1 pad 181: (no net) -> /181
- X1 pad 182: (no net) -> /182
- X1 pad 183: (no net) -> /183
- X1 pad 184: (no net) -> /184
- X1 pad 185: (no net) -> /185
- X1 pad 186: (no net) -> /186
- X1 pad 187: (no net) -> /187
- X1 pad 188: (no net) -> /188
- X1 pad 189: (no net) -> /189
- X1 pad 19: (no net) -> /19
- X1 pad 190: (no net) -> /190
- X1 pad 191: (no net) -> /191
- X1 pad 192: (no net) -> /192
- X1 pad 193: (no net) -> /193
- X1 pad 194: (no net) -> /194
- X1 pad 195: (no net) -> /195
- X1 pad 196: (no net) -> /196
- X1 pad 197: (no net) -> /197
- X1 pad 198: (no net) -> /198
- X1 pad 199: (no net) -> /199
- X1 pad 2: (no net) -> /2
- X1 pad 20: (no net) -> /20
- X1 pad 200: (no net) -> /200
- X1 pad 201: (no net) -> /201
- X1 pad 202: (no net) -> /202
- X1 pad 203: (no net) -> /203
- X1 pad 204: (no net) -> /204
- X1 pad 205: (no net) -> /205
- X1 pad 206: (no net) -> /206
- X1 pad 207: (no net) -> /207
- X1 pad 208: (no net) -> /208
- X1 pad 209: (no net) -> /209
- X1 pad 21: (no net) -> /21
- X1 pad 210: (no net) -> /210
- X1 pad 211: (no net) -> /211
- X1 pad 212: (no net) -> /212
- X1 pad 213: (no net) -> /213
- X1 pad 214: (no net) -> /214
- X1 pad 215: (no net) -> /215
- X1 pad 216: (no net) -> /216
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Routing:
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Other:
- board outline added: 136 x 152 mm
- net class Default: clearance 0.2 -> 0.125; trace_width 0.25 -> 0.125; via_dia 0.8 -> 0.6; via_drill 0.4 -> 0.3
- rule trace_clearance: 0.2 -> 0.125
- rule trace_min: 0.2 -> 0.125
- rule via_min_size: 0.4 -> 0.6
